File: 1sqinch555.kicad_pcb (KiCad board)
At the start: 2 copper layers, 104.5 x 25 mm, 84 parts, among them J1 Conn_01x01, J10 Conn_01x01, J11 Conn_01x01, J12 Conn_01x01, J13 Conn_01x01, J14 Conn_01x01, J15 Conn_01x01, J16 Conn_01x01, J17 Conn_01x01, J18 Conn_01x01, J19 Conn_01x01, J2 Conn_01x01, J20 Conn_01x01, J21 Conn_01x01, J22 Conn_01x01, J23 Conn_01x01, J24 Conn_01x01, J25 Conn_01x01, J26 Conn_01x01, J27 Conn_01x01, J28 Conn_01x01, J29 Conn_01x01, J3 Conn_01x01, J30 Conn_01x01, J31 Conn_01x01, J32 Conn_01x01, J33 Conn_01x01, J34 Conn_01x01, J35 Conn_01x01, J4 Conn_01x01, J5 Conn_01x01, J6 Conn_01x01, J7 Conn_01x01, J8 Conn_01x01, J9 Conn_01x01, U1 LM555, U2 4020

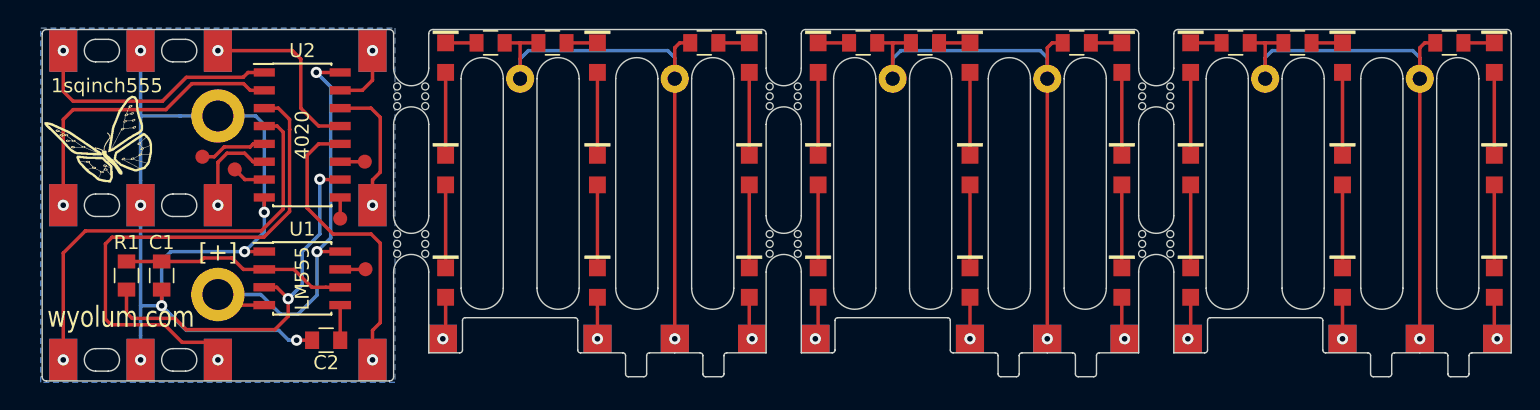
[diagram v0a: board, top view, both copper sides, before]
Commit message: mods
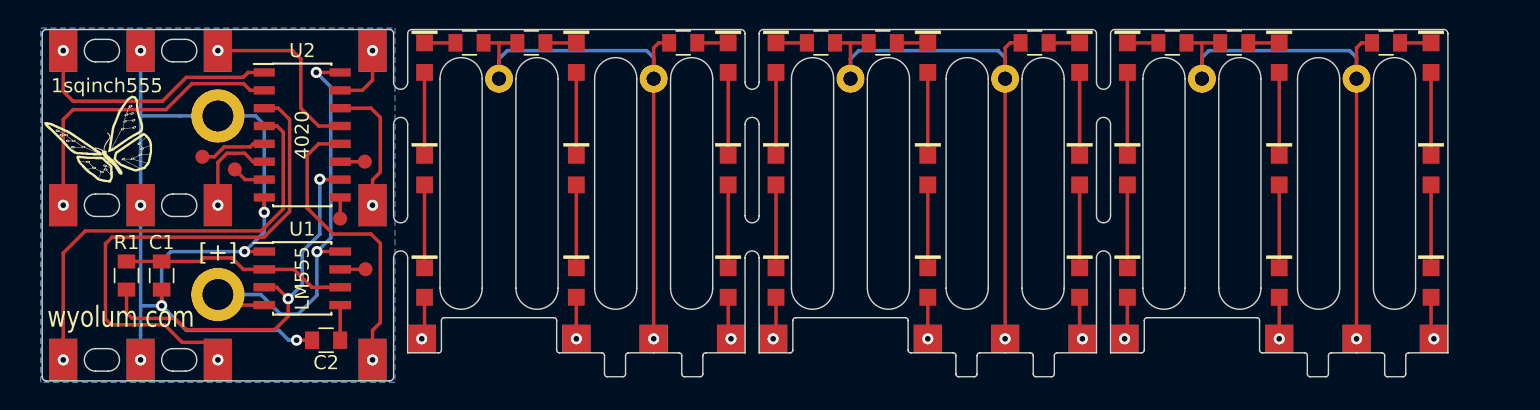
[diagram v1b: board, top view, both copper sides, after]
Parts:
- removed mouse-bite-2.5mm-slot (x6): VAL**, 1sqinch555_fp:mouse-bite-2.5mm-slot
- moved D19 4.50 mm to (114.7, 55.5)
- moved D20 4.50 mm to (114.7, 47.5)
- moved D21 4.50 mm to (114.7, 39.5)
- moved D22 4.50 mm to (125.5, 55.5)
- moved D23 4.50 mm to (125.5, 47.5)
- moved D24 4.50 mm to (125.5, 39.5)
- moved D25 4.50 mm to (136.3, 55.5)
- moved D26 4.50 mm to (136.3, 47.5)
- moved D27 4.50 mm to (136.3, 39.5)
- moved J19 4.50 mm to (114.5, 59.5)
- moved J21 4.50 mm to (125.5, 59.5)
- moved J23 4.50 mm to (136.5, 59.5)
- moved J29 4.50 mm to (131.0, 59.5)
- moved J34 4.50 mm to (131.0, 41.0)
- moved J35 4.50 mm to (120.0, 41.0)
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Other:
- board size 104.5 x 25 mm -> 100 x 25 mm
